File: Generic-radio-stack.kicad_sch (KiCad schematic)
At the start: 14 parts, among them J1 USB_B_Mini, U1 NCP1117-3.3_SOT223

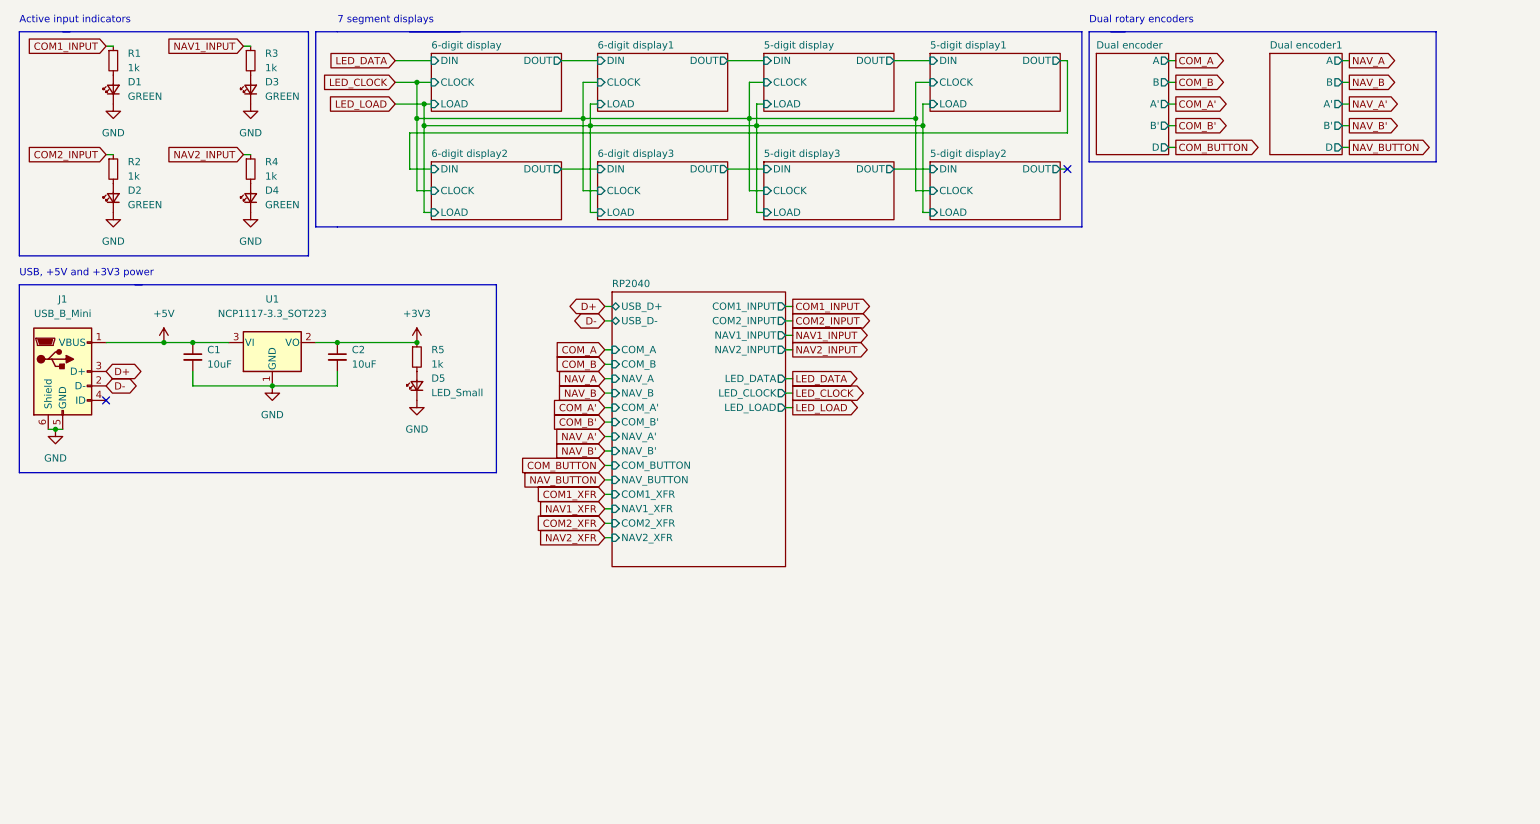
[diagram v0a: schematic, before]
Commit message: Bunch more schematic work
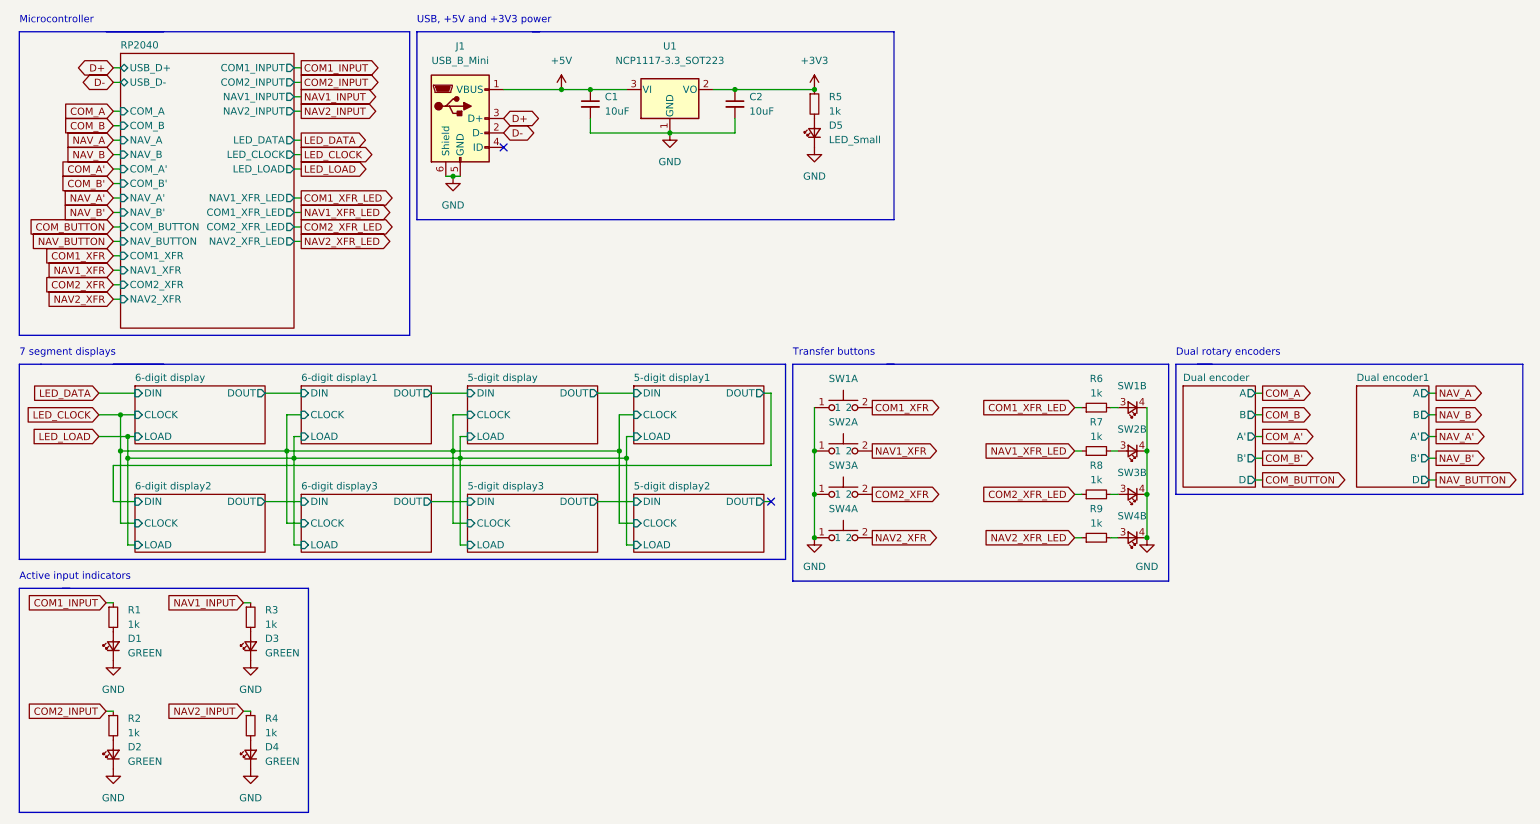
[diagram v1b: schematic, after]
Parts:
- added R6, R7, R8, R9: 1k, Resistor_SMD:R_0805_2012Metric, symbol Device:R_Small
- added SW1, SW2, SW3, SW4: SW_Push_LED, Generic-radio-stack:SW_PUSH_6mm, symbol Generic-radio-stack:SW_Push_LED
- D1, D2, D3, D4: footprint (none) -> LED_THT:LED_D5.0mm
- D5: footprint (none) -> Generic-radio-stack:LED_0603_1608Metric
- J1: footprint (none) -> Generic-radio-stack:USB_B_Mini_Amphenol_UE25BE5510H
- R1, R2, R3, R4, R5: footprint (none) -> Resistor_SMD:R_0805_2012Metric
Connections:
- net COM1_XFR: now also SW1.2
- net COM2_XFR: now also SW3.2
- net GND: now also SW1.1, SW1.4, SW2.1, SW2.4, SW3.1, SW3.4, SW4.1, SW4.4
- net NAV1_XFR: now also SW2.2
- net NAV2_XFR: now also SW4.2
- new net: R9.2, SW4.3
- new net: R8.2, SW3.3
- new net: R6.2, SW1.3
- new net: R7.2, SW2.3
- new net COM1_XFR_LED: R6.1
- new net COM2_XFR_LED: R8.1
- new net NAV1_XFR_LED: R7.1
- new net NAV2_XFR_LED: R9.1
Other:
- sheet RP2040 ports: added COM1_XFR_LED, COM2_XFR_LED, NAV1_XFR_LED, NAV2_XFR_LED; removed none
- note added: "Microcontroller"
- note added: "Transfer buttons"
- moved on the sheet: C1, C2, D1, D2, D3, D4, D5, J1, R1, R2, R3, R4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
